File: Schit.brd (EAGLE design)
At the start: 58.1 x 47 mm, 15 parts, among them IC2 MEGA16-A, Q1 12M

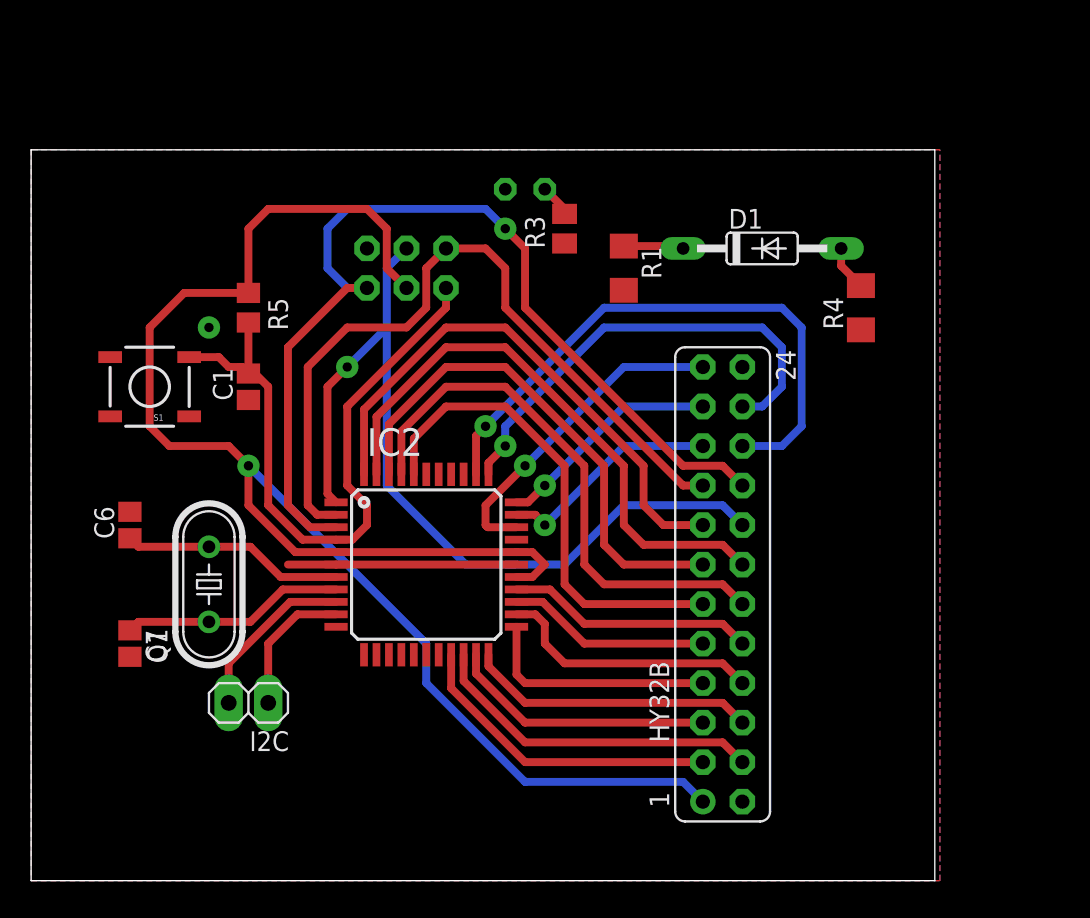
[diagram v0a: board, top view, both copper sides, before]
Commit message: 1.0.1
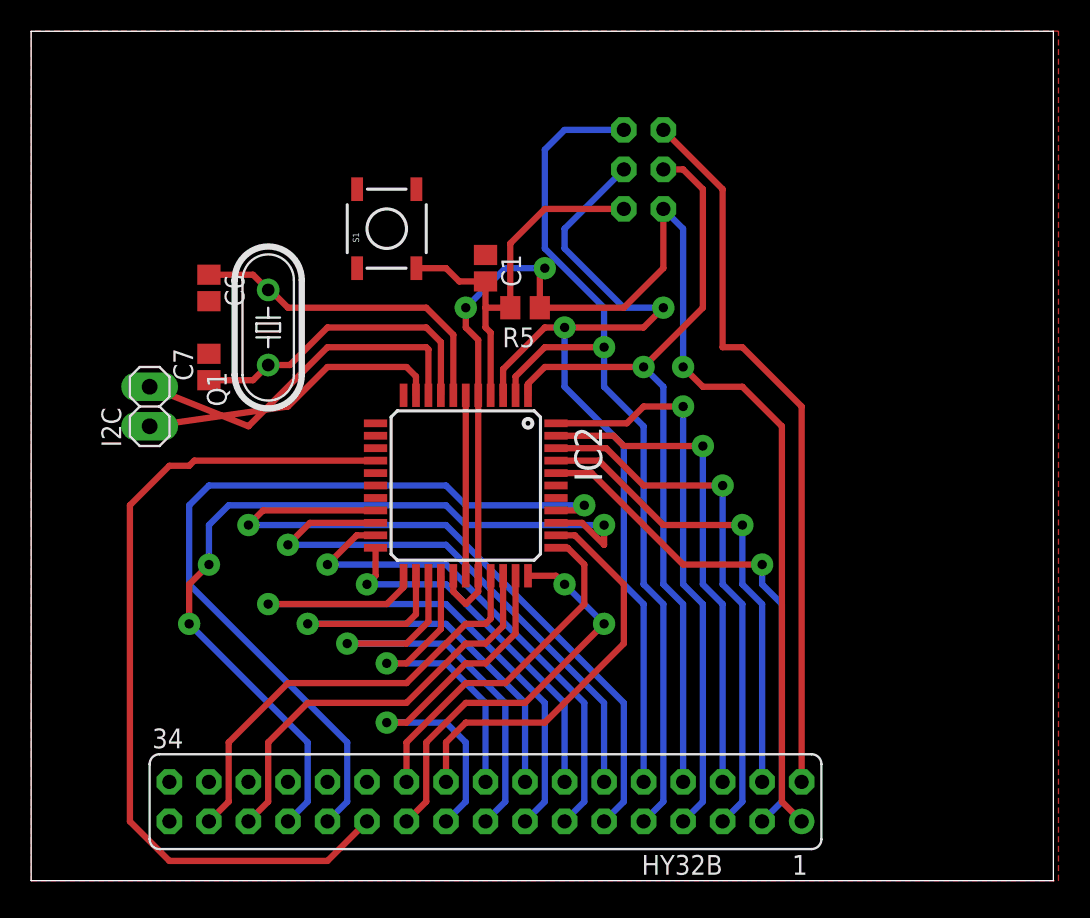
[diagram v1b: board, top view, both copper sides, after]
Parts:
- removed D1: 1N4446, diode:DO35-10
- removed R1: 220, resistor:R1206
- removed R3: 220, rcl:M2012
- removed R4: 20, resistor:R1206
- removed STAT_LED: (no value), led:LED3MM
- HY32B: device con-lsta:FE12-2 -> con-lsta:FE17-2
- moved HY32B 20.7 mm to (29.2, 5.08), turned to 180 degrees
- moved I2C 20.1 mm to (7.62, 30.5), turned to 90 degrees
- moved C7 18.5 mm to (11.4, 33.0), turned to 90 degrees
- moved S1 18.3 mm to (22.9, 41.9), turned to 90 degrees
- moved R5 17.8 mm to (31.8, 36.8), turned to 180 degrees
- moved C1 17.0 mm to (29.2, 39.4), turned to 270 degrees
- moved Q1 16.9 mm to (15.2, 35.6)
- moved SPI 16.5 mm to (39.4, 45.7), turned to 90 degrees
- moved C6 16.1 mm to (11.4, 38.1), turned to 270 degrees
- moved IC2 5.68 mm to (27.9, 25.4), turned to 270 degrees
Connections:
- removed net D5: HY32B.8, IC2.24
- removed net D6: HY32B.9, IC2.25
- removed net D7: HY32B.10, IC2.26
- removed net N$1: D1.C, R1.1
- removed net N$13: IC2.15
- removed net N$2: D1.A, R4.2
- removed net N$42: IC2.30
- removed net N$9: R3.2, STAT_LED.A
- new net BL_CNT: HY32B.24
- new net D5_SPI_MOSI: HY32B.8, IC2.1, SPI.4
- new net D6_SPI_MISO: HY32B.9, IC2.2, SPI.5
- new net D7_SPI_SCK: HY32B.10, IC2.3, SPI.3
- new net N$21: HY32B.34
- new net N$22: HY32B.33
- new net NC: HY32B.28, HY32B.30, HY32B.32
- new net TPCS: HY32B.31, IC2.30
- new net TP_IRQ: HY32B.26
- new net TP_SCK: HY32B.29, IC2.31
- new net TP_SI: HY32B.27, IC2.36
- new net TP_SO: HY32B.25, IC2.37
- net D0: now also IC2.40; no longer IC2.19
- net D1: now also IC2.41; no longer IC2.20
- net D10: now also IC2.21; no longer IC2.42
- net D11: now also IC2.22; no longer IC2.43
- net D12: now also IC2.23; no longer IC2.44
- net D13: now also IC2.24; no longer IC2.1, SPI.4
- net D14: now also IC2.25; no longer IC2.2, SPI.2
- net D15: now also IC2.26; no longer IC2.3, SPI.5
- net D2: now also IC2.42; no longer IC2.21
- net D3: now also IC2.43; no longer IC2.22
- net D4: now also IC2.44; no longer IC2.23
- net D8: now also IC2.19; no longer IC2.40
- net D9: now also IC2.20; no longer IC2.41
- net GND: no longer R4.1, STAT_LED.K
- net RST: now also IC2.15; no longer IC2.31
- net VCC: now also SPI.2; no longer SPI.3
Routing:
- net D6_SPI_MISO: track 0.00 -> 60.1 mm, vias 0 -> 1
- net D7_SPI_SCK: track 0.00 -> 59.5 mm, vias 0 -> 2
- net TP_SI: track 0.00 -> 54.7 mm, vias 0 -> 3
- net TP_SO: track 0.00 -> 53.5 mm, vias 0 -> 1
- net D5_SPI_MOSI: track 0.00 -> 52.4 mm, vias 0 -> 1
- net GND: track 14.7 -> 57.9 mm, vias 1 -> 0
- net D15: track 62.9 -> 20.3 mm
- net RST: track 21.0 -> 54.6 mm, vias 1 -> 0
- net TPCS: track 0.00 -> 28.5 mm
- net TP_SCK: track 0.00 -> 27.0 mm
- net D13: track 55.9 -> 30.8 mm
- net D4: track 15.3 -> 36.3 mm, vias 0 -> 1
- net D14: track 48.8 -> 28.6 mm, vias 0 -> 1
- net D2: track 17.1 -> 34.3 mm, vias 0 -> 1
- net D5: track 17.1 -> 0.00 mm
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- removed copper zone on layer 16, net GND
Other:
- board size 58.1 x 47 mm -> 65.7 x 54.6 mm
